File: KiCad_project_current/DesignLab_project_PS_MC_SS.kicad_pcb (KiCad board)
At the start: 2 copper layers, 133.5 x 89 mm, 61 parts, among them J1 Conn_01x09, J2 USB_B_Micro, J3 Barrel_Jack, J4 Conn_02x08_Odd_Even, SW1 SW_Push, SW2 SW_Push, SW3 SW_Push, SW4 SW_Push, SW5 SW_Push, U1 ATmega328P-P, U2 CH340C, U3 BMP280, U4 DS18B20, U5 L7805, U6 LTC-4627JD, U7 LM1117DT-3.3, Y1 16MHz

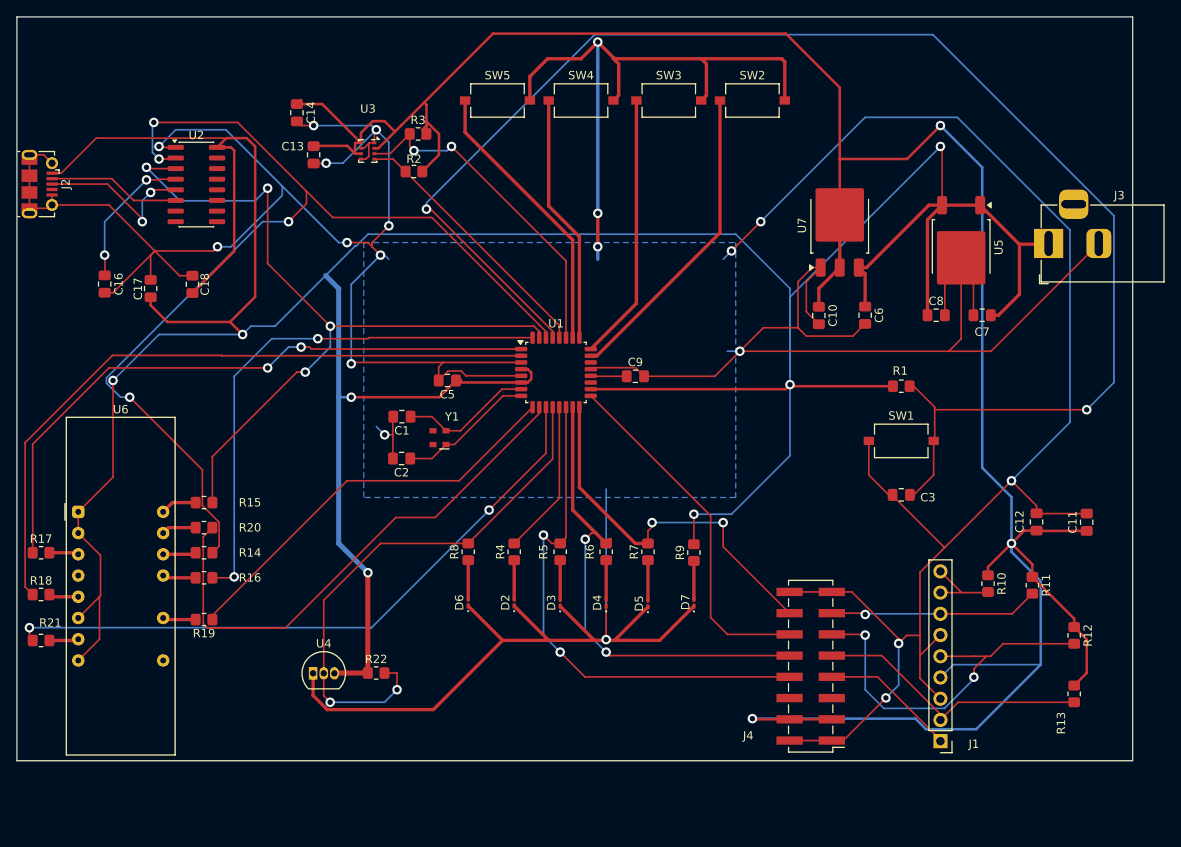
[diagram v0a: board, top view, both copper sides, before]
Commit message: Current version of KiCad project
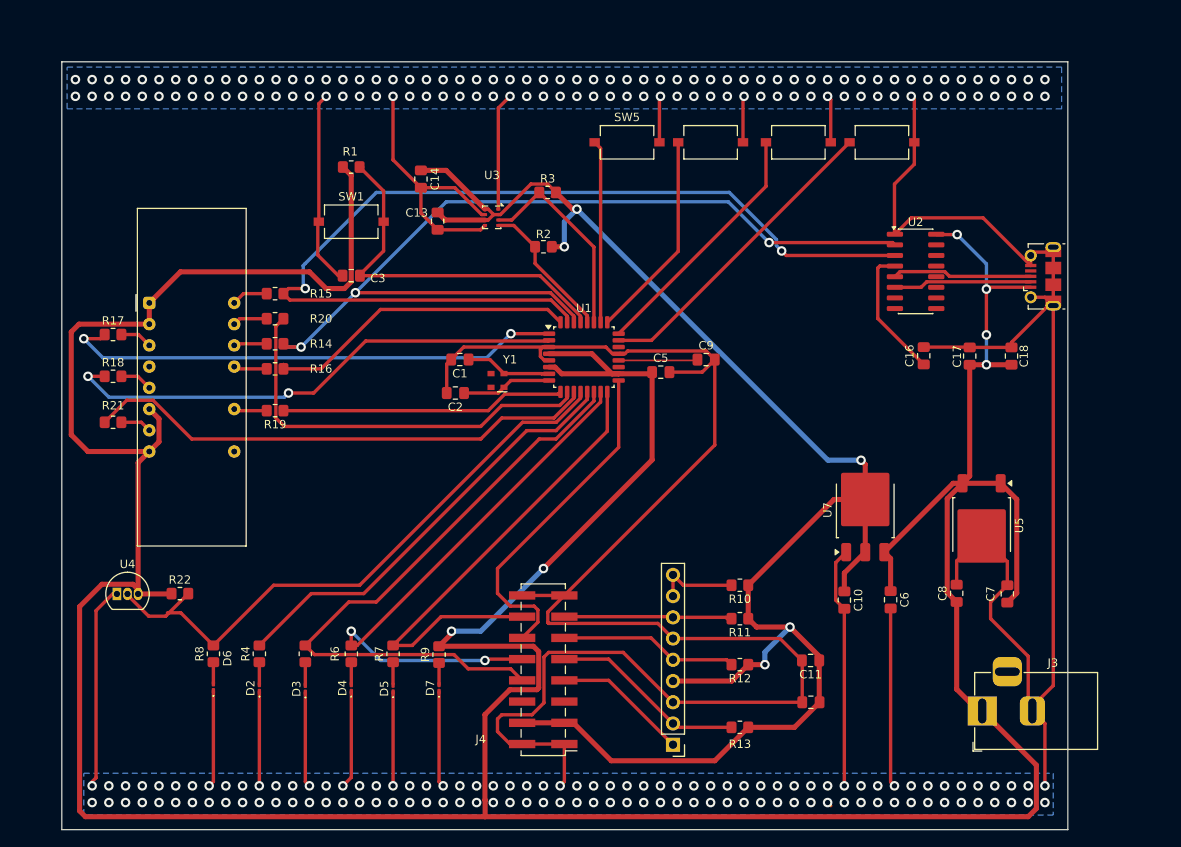
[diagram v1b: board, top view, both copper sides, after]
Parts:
- moved J2 120.5 mm to (241.3, 62.5), turned to 90 degrees
- moved C16 98.4 mm to (227.0, 72.0), turned to 90 degrees
- moved C18 98.4 mm to (237.5, 72.1)
- moved C17 98.3 mm to (232.5, 72.1)
- moved U2 86.7 mm to (226.0, 61.9)
- moved C3 70.8 mm to (158.5, 62.5)
- moved R1 70.8 mm to (158.5, 49.5)
- moved SW1 70.8 mm to (158.5, 56.0)
- moved J3 56.5 mm to (234.0, 114.5)
- moved R13 40.2 mm to (205.0, 116.5), turned to 180 degrees
- moved R12 40.2 mm to (205.0, 109.0), turned to 180 degrees
- moved C11 36.9 mm to (213.5, 108.5), turned to 180 degrees
- moved R11 35.2 mm to (205.0, 103.5), turned to 180 degrees
- moved C12 34.6 mm to (213.5, 113.5), turned to 180 degrees
- moved C10 34.2 mm to (217.5, 101.3)
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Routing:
- net RESET: track 180.6 -> 45.2 mm, vias 2 -> 0
- net +3.3V: track 308.8 -> 197.8 mm, vias 3 -> 5
- net GND: track 693.0 -> 586.0 mm, vias 20 -> 234
- net PB1: track 18.5 -> 52.3 mm
- net PD2: track 64.9 -> 37.4 mm, vias 2 -> 0
- net TX/PD1: track 93.5 -> 119.5 mm, vias 4 -> 2
- net SCK: track 46.3 -> 21.3 mm, vias 2 -> 0
- net PD4: track 82.2 -> 61.0 mm, vias 0 -> 2
- net PC4: track 40.7 -> 24.5 mm, vias 2 -> 0
- net PD3: track 76.4 -> 60.5 mm
- net PD7: track 77.6 -> 62.5 mm, vias 2 -> 0
- net PC5: track 31.9 -> 17.1 mm
- net PD5: track 49.1 -> 34.6 mm
- net PD6: track 63.7 -> 49.7 mm
- net PB2: track 62.5 -> 75.4 mm, vias 2 -> 0
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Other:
- board size 133.5 x 89 mm -> 120.4 x 91.9 mm
